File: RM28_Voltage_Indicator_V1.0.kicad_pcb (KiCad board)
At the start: 2 copper layers, 33.9 x 21.8 mm, 18 parts, among them IC1 NCP785AH120T1G, J1 649002227222, J2 649002227222, Q1 SBCP56-16T1G, U1 1SMB5927BT3G

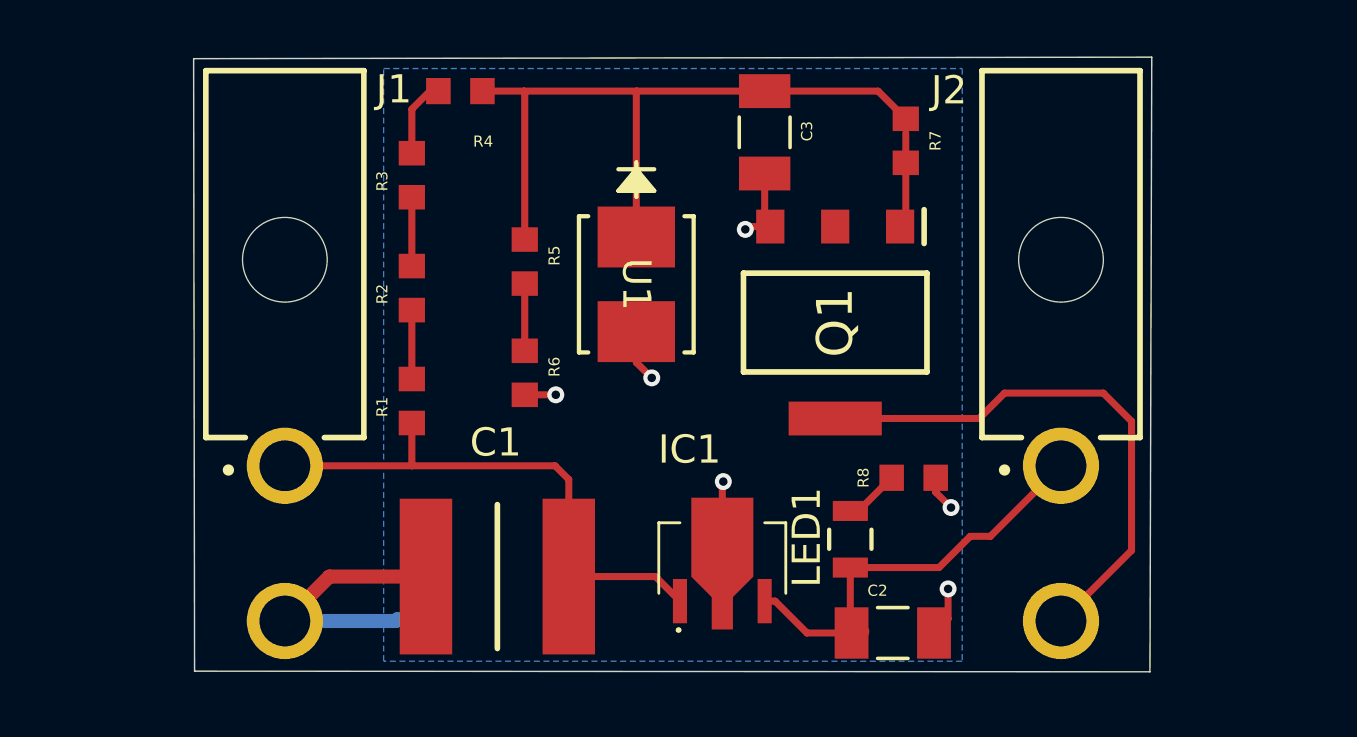
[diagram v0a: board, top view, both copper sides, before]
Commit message: Final changes for layout
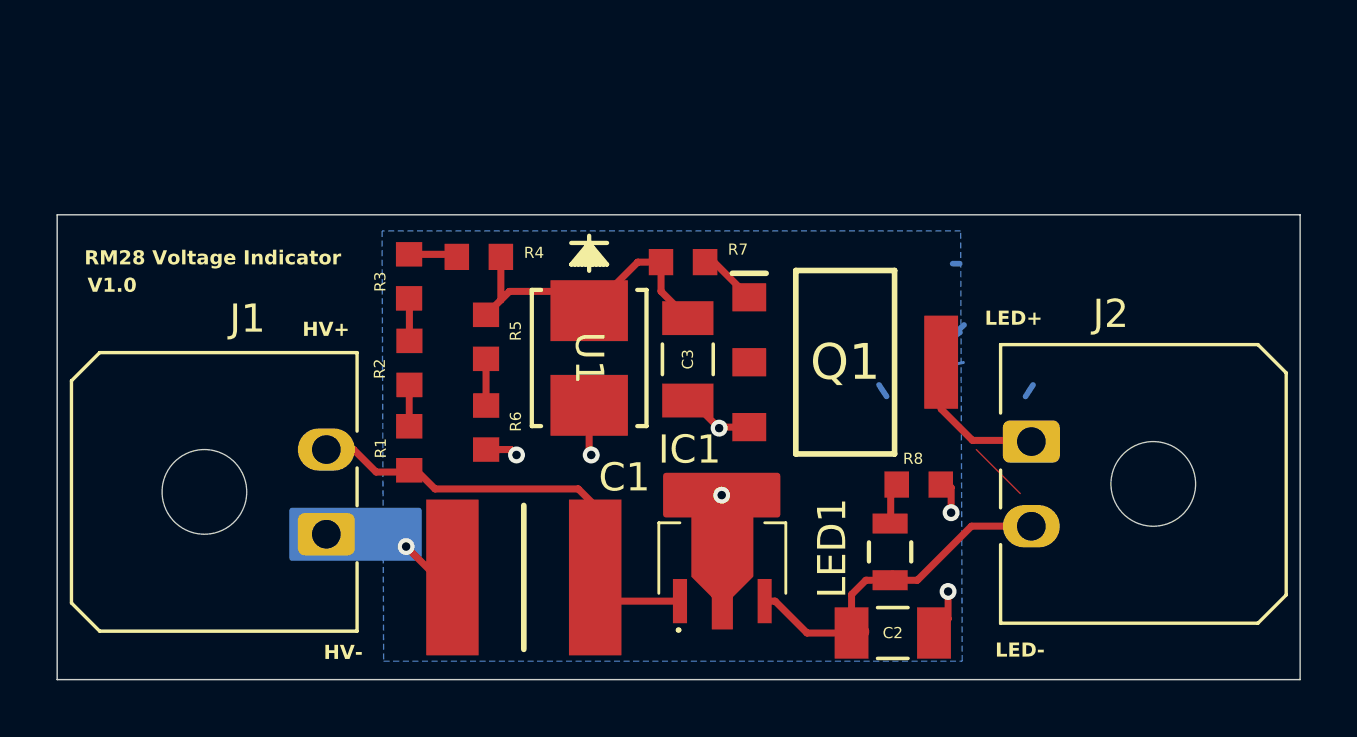
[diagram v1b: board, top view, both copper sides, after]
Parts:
- added REF**: Symbol_HighVoltage_Triangle_6x6mm_Copper, Symbol:Symbol_HighVoltage_Triangle_6x6mm_Copper, B.Cu at (126.3, 59.1)
- added REF**: OSHW-Logo2_7.3x6mm_SilkScreen, Symbol:OSHW-Logo2_7.3x6mm_SilkScreen, B.Cu at (133.4, 59.9)
- added REF**: ESD-Logo_6.6x6mm_SilkScreen, Symbol:ESD-Logo_6.6x6mm_SilkScreen, B.Cu at (99.2, 59.5)
- J1, J2: value 649002227222 -> Molex_Micro-Fit_3.0_43650-0200_1x02_P3.00mm_Horizontal; footprint 649002227222:649002227222 -> Connector_Molex:Molex_Micro-Fit_3.0_43650-0200_1x02_P3.00mm_Horizontal
- moved G*** 12.7 mm to (114.5, 68.3)
- moved J1 10.0 mm to (104.0, 66.5), turned to 90 degrees
- moved R7 8.99 mm to (116.6, 56.9), turned to 0 degrees
- moved C3 8.49 mm to (116.8, 60.3)
- moved J2 6.72 mm to (128.9, 63.2), turned to -90 degrees
- moved R4 5.91 mm to (109.4, 56.7)
- moved R3 3.58 mm to (106.9, 57.4)
- moved U1 3.10 mm to (113.3, 60.3)
- moved R5 3.00 mm to (109.6, 59.5)
- moved R2 2.65 mm to (106.9, 60.4)
- moved R6 2.37 mm to (109.6, 62.7)
- moved R1 1.68 mm to (106.9, 63.5)
- moved LED1 1.48 mm to (123.9, 67.1)
- moved Q1 1.45 mm to (122.4, 60.4), turned to 0 degrees
- moved C1 0.94 mm to (111.0, 68.0)
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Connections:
- J1 pad 1: /+HV -> GND
- J1 pad 2: GND -> /+HV
- J2 pad 1: Net-(IC1-VOUT) -> Net-(Q1-C_2)
- J2 pad 2: Net-(Q1-C_2) -> Net-(IC1-VOUT)
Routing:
- net Net-(Q1-C_2): track 19.4 -> 4.93 mm
- net Net-(U1-CATHODE): track 25.9 -> 11.4 mm
- net GND: track 23.4 -> 12.8 mm, vias 6 -> 7
- net /+HV: track 19.5 -> 16.3 mm
- net (no net): track 0.00 -> 2.20 mm
- net Net-(IC1-VOUT): track 15.0 -> 13.2 mm
- net Net-(Q1-B): track 3.40 -> 2.08 mm
- net Net-(R3-Pad2): track 2.77 -> 1.73 mm
- net Net-(R1-Pad2): track 2.44 -> 1.47 mm
- net Net-(R2-Pad2): track 2.44 -> 1.51 mm
- net Net-(R5-Pad2): track 2.38 -> 1.66 mm
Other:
- board size 33.9 x 21.8 mm -> 44 x 16.5 mm
- board text added: "Das Rennwagen ist schnell - S.C.T."
- board text added: "HV+"
- board text added: "HV-"
- board text added: "LED+"
- board text added: "LED-"
- board text added: "RM28 Voltage Indicator"
- board text added: "V1.0"
